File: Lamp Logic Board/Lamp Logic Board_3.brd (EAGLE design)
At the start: 41.5 x 84.8 mm, 45 parts, among them U1 ESP32-WROVER-IB, U2 SN74HCT245DWR, U4 LM50, U5 SPIOLED_STANDOFF, U6 MSGEQ7DIL

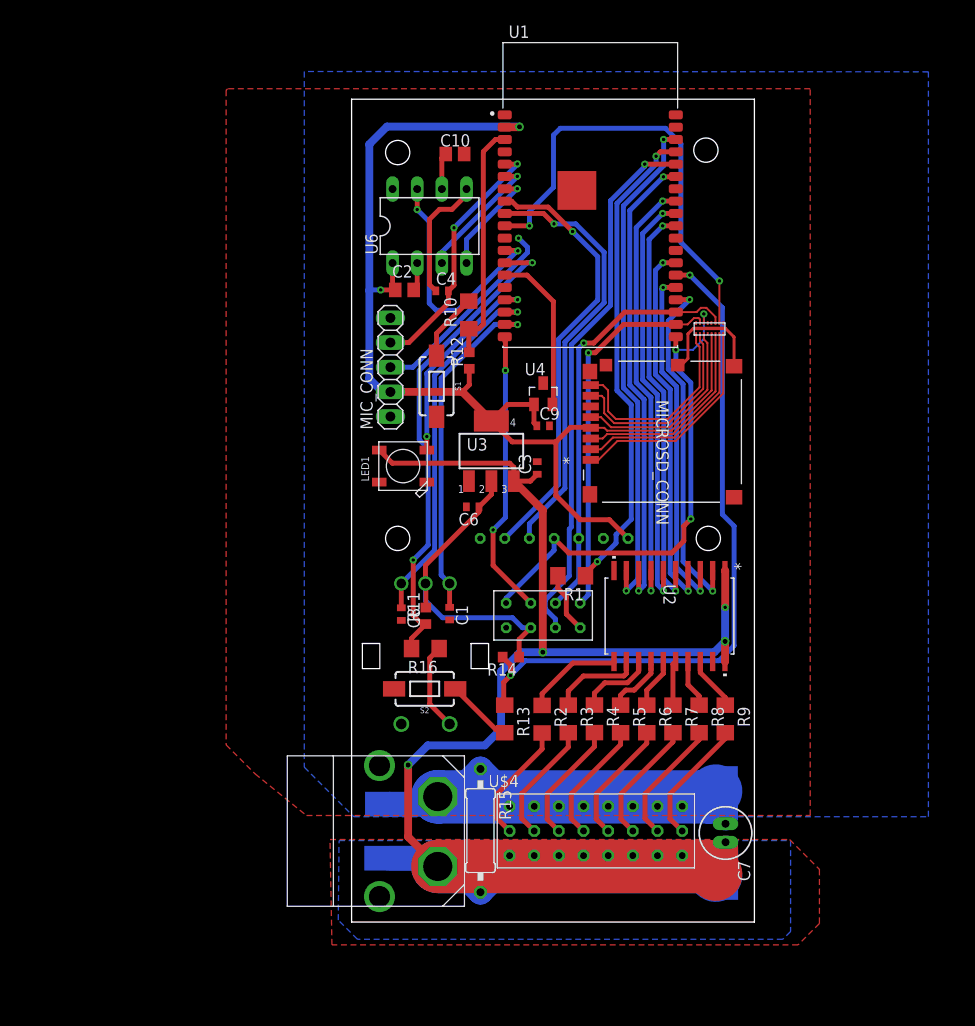
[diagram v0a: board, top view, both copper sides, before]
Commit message: Another day closer to death...
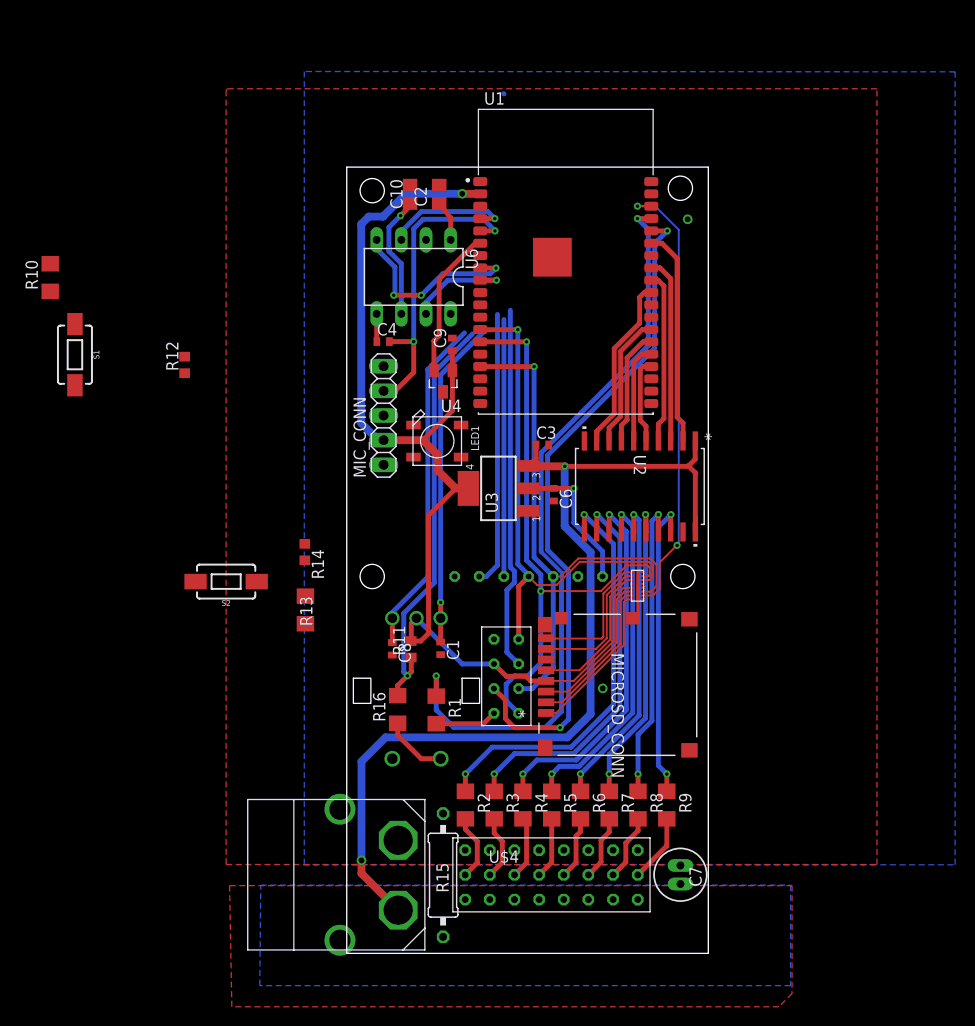
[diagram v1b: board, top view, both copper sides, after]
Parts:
- removed PAD5V, PAD5V1, PADGND, PADGND1: (no value), wirepad:SMD2,54-5,08
- moved R10 43.3 mm to (-30.6, 69.6)
- moved S1 37.4 mm to (-28.0, 61.7)
- moved R12 29.3 mm to (-16.7, 60.6)
- moved MICROSD_CONN 26.5 mm to (27.9, 27.7)
- moved U$3 25.2 mm to (29.4, 39.5), turned to 270 degrees
- moved R14 23.8 mm to (-4.32, 41.3), turned to 270 degrees
- moved R13 23.4 mm to (-4.25, 35.4)
- moved S2 23.2 mm to (-12.4, 38.3)
- moved R1 19.6 mm to (9.22, 25.1), turned to 270 degrees
- moved U2 13.7 mm to (30.2, 48.1)
- moved C9 12.6 mm to (10.9, 62.7), turned to 90 degrees
- moved R2 11.9 mm to (12.2, 15.3)
- moved R3 11.7 mm to (15.2, 15.3)
- moved R4 11.5 mm to (18.2, 15.3)
- moved R5 11.4 mm to (21.1, 15.3)
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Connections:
- new net N$30: U1.37
- new net N$38: U1.20
- new net N$39: U1.19
- new net N$40: U1.18
- new net N$41: U1.17
- new net N$42: U1.22
- new net N$43: U1.21
- net CS: no longer U1.19
- net GAIN: no longer U1.11
- net GND: no longer PADGND.1, PADGND1.1
- net IO0: no longer U1.25
- net LEDS1_3V3: now also U1.33; no longer U1.23
- net LEDS2_3V3: now also U1.31; no longer U1.24
- net LEDS3_3V3: now also U1.30; no longer U1.26
- net LEDS4_3V3: now also U1.23; no longer U1.29
- net LEDS5_3V3: now also U1.24; no longer U1.30
- net LEDS6_3V3: now also U1.25; no longer U1.31
- net LEDS7_3V3: now also U1.26; no longer U1.33
- net LEDS8_3V3: now also U1.29; no longer U1.36
- net LEDSDIAG_3V3: no longer U1.16
- net MISO: now also U1.14; no longer U1.21
- net MOSI: now also U1.16; no longer U1.22
- net MSGEQ_OUT: now also U1.4; no longer U1.6
- net MSGEQ_RST: now also U1.9; no longer U1.12
- net MSGEQ_STROBE: now also U1.8; no longer U1.7
- net OLED_CS: no longer U1.9
- net OLED_DC: no longer U1.8
- net OUTA: now also U1.10, U1.7; no longer U1.17
- net OUTB: now also U1.12; no longer U1.18
- net ROTARY_BUTTON_IN: now also U1.11; no longer U1.13
- net SCK: now also U1.13; no longer U1.20
- net SD_CS: now also U1.36; no longer U1.10
- net VDD3V3_TEMP_OUT: now also U1.6; no longer U1.14
- net VDD5V: no longer PAD5V.1, PAD5V1.1
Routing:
- net VDD5V: track 236.2 -> 99.8 mm, vias 4 -> 2
- net GND: track 97.0 -> 3.57 mm, vias 0 -> 2
- net IO0: track 71.9 -> 0.00 mm, vias 2 -> 0
- net LEDS8_3V3: track 52.7 -> 18.0 mm, vias 2 -> 0
- net LEDS7_3V3: track 48.3 -> 13.8 mm, vias 2 -> 0
- net LEDS4_3V3: track 42.8 -> 8.91 mm, vias 2 -> 0
- net LEDS5_3V3: track 44.1 -> 10.3 mm, vias 2 -> 0
- net LEDS6_3V3: track 45.4 -> 12.0 mm, vias 2 -> 0
- net N$15: track 10.1 -> 42.6 mm, vias 0 -> 2
- net N$14: track 10.0 -> 40.2 mm, vias 0 -> 2
- net N$13: track 7.74 -> 37.8 mm, vias 0 -> 2
- net N$12: track 6.31 -> 35.4 mm, vias 0 -> 2
- net N$2: track 49.7 -> 78.1 mm
- net N$11: track 5.20 -> 33.0 mm, vias 0 -> 2
- net N$10: track 4.61 -> 31.9 mm, vias 0 -> 2
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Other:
- board size 41.5 x 84.8 mm -> 37.2 x 81 mm
